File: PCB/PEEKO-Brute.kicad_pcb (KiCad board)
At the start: 2 copper layers, 52.1 x 45.7 mm, 61 parts, among them J1 Rasberry PI Pico, J2 Conn_02x15_Odd_Even, J3 Conn_01x02_Pin, J4 Conn_01x02_Pin

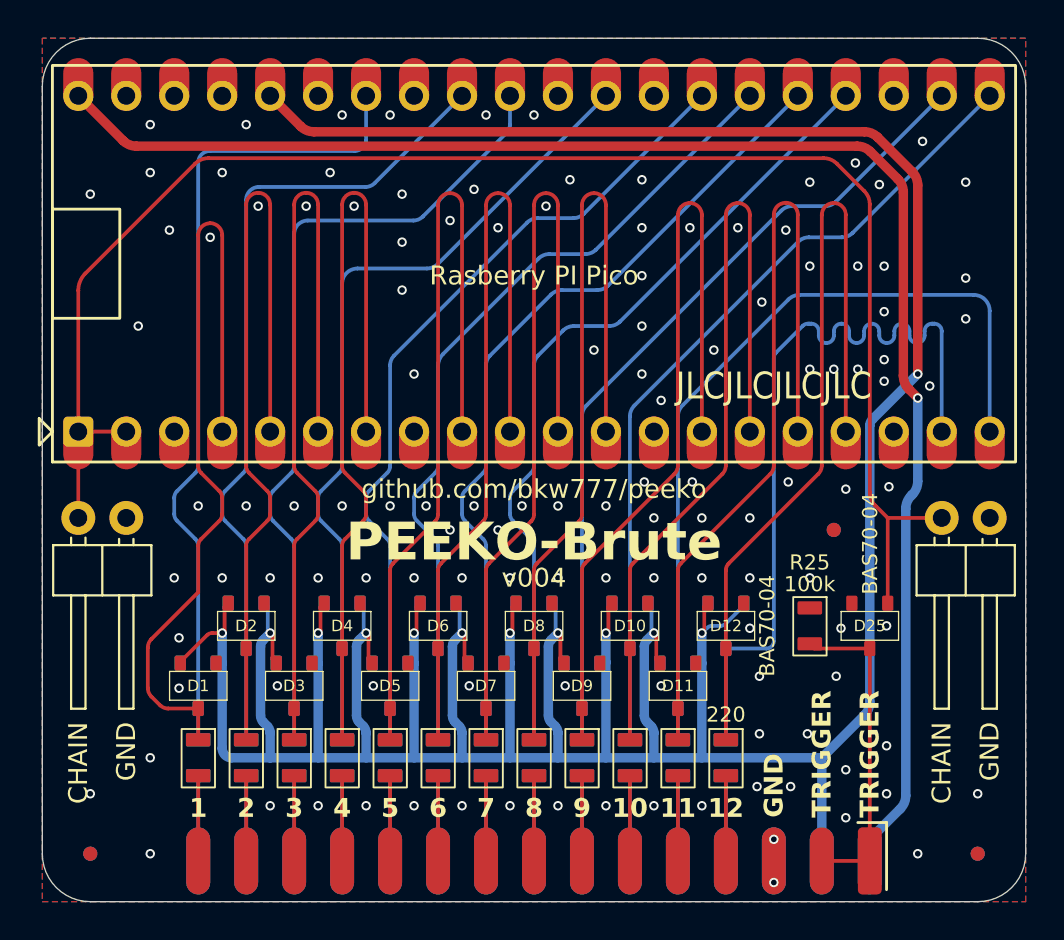
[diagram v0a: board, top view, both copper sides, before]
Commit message: make brute the same dimensions and port placement as regular peeko, use same housing for both
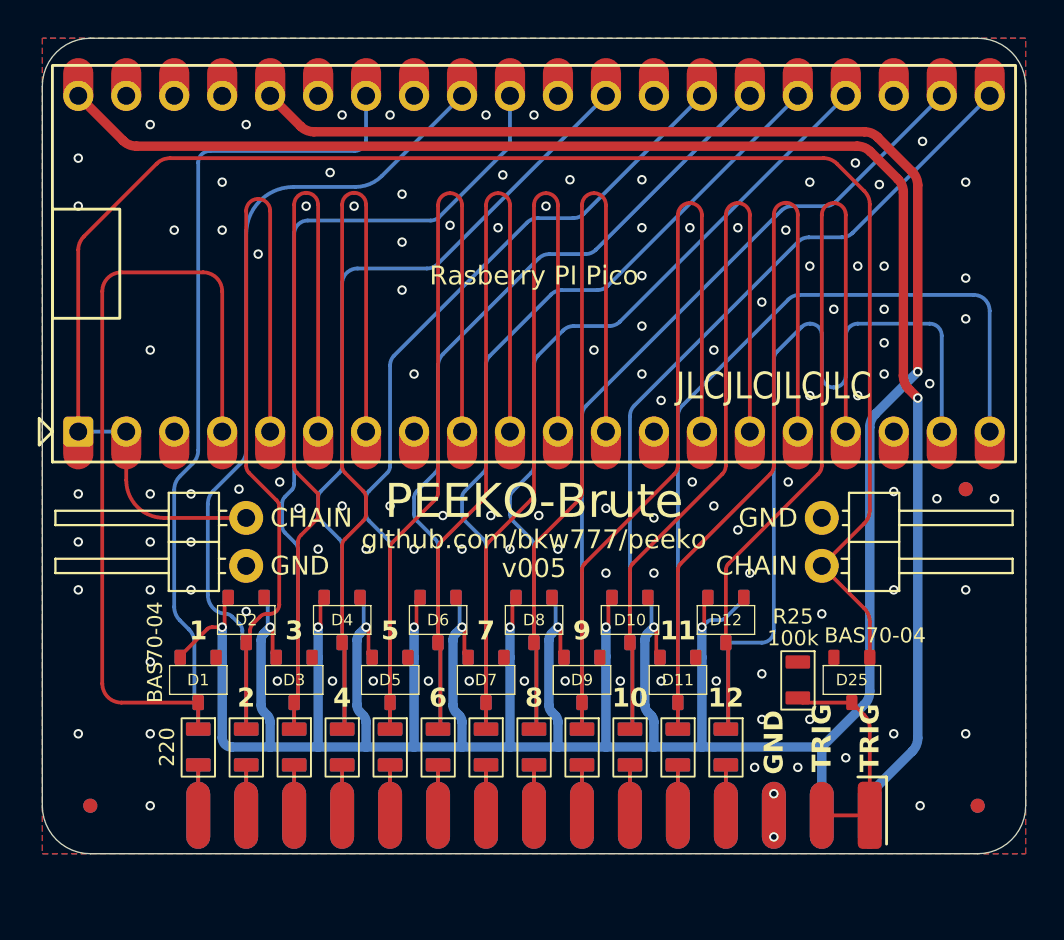
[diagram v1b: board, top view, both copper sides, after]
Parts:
- N1: value PEEKO-Brute Housing -> PEEKO Housing; footprint 000_LOCAL:PEEKO-Brute_housing -> 000_LOCAL:PEEKO_housing
- moved J3 8.89 mm to (161.3, 108.2), turned to 0 degrees
- moved REF** 7.31 mm to (168.9, 106.7) (x2)
- moved J4 6.84 mm to (130.8, 110.7), turned to 180 degrees
- moved D25 3.02 mm to (162.8, 116.8)
- moved R25 2.93 mm to (160.0, 116.8)
- moved REF** 2.54 mm to (122.5, 123.4) (x2)
- moved REF** 2.54 mm to (169.5, 123.4) (x2)
- moved J2 2.41 mm to (146.0, 126.1)
- moved N1 1.27 mm to (146.0, 104.4)
- moved R1 0.57 mm to (128.2, 120.3)
- moved R10 0.57 mm to (151.1, 120.3)
- moved R11 0.57 mm to (153.6, 120.3)
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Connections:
- J2 pad 3: unconnected-(J2-Pin_3-Pad3) -> /TRIGGER
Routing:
- net /CHAIN: track 85.1 -> 93.4 mm
- net +3V3: track 215.5 -> 210.1 mm
- net /TRIGGER: track 17.1 -> 12.2 mm
- net +5V: track 82.5 -> 80.2 mm
- net /CH9: track 4.51 -> 2.67 mm
- net /CH8: track 4.51 -> 2.67 mm
- net /CH7: track 4.51 -> 2.67 mm
- net /CH6: track 4.51 -> 2.67 mm
- net /CH5: track 4.51 -> 2.67 mm
- net /CH4: track 4.51 -> 2.67 mm
- net /CH3: track 4.51 -> 2.67 mm
- net /CH23: track 4.51 -> 2.67 mm
- net /CH22: track 4.51 -> 2.67 mm
- net /CH21: track 4.51 -> 2.67 mm
- net /CH20: track 4.51 -> 2.67 mm
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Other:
- board size 52.1 x 45.7 mm -> 52.1 x 43.2 mm
- board text added: "TRIG"
- board text added: "trace lengths 38.16 + 4.58 = 42.74 41.34 + 1.40 = 42.74"
- board text removed: "TRIGGER"
- board text removed: "trace lengths 38.46 + 4.84 = 43.3 41.64 + 1.66 = 43.3"
